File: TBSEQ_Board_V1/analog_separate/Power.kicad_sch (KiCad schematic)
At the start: 7 parts, among them IC11 AN6562, IC12 4066, J1 Conn_01x03_Pin, J3 Conn_01x03_Pin, J4 Conn_01x03_Pin, J5 Conn_01x03_Pin, J6 Conn_01x03_Pin

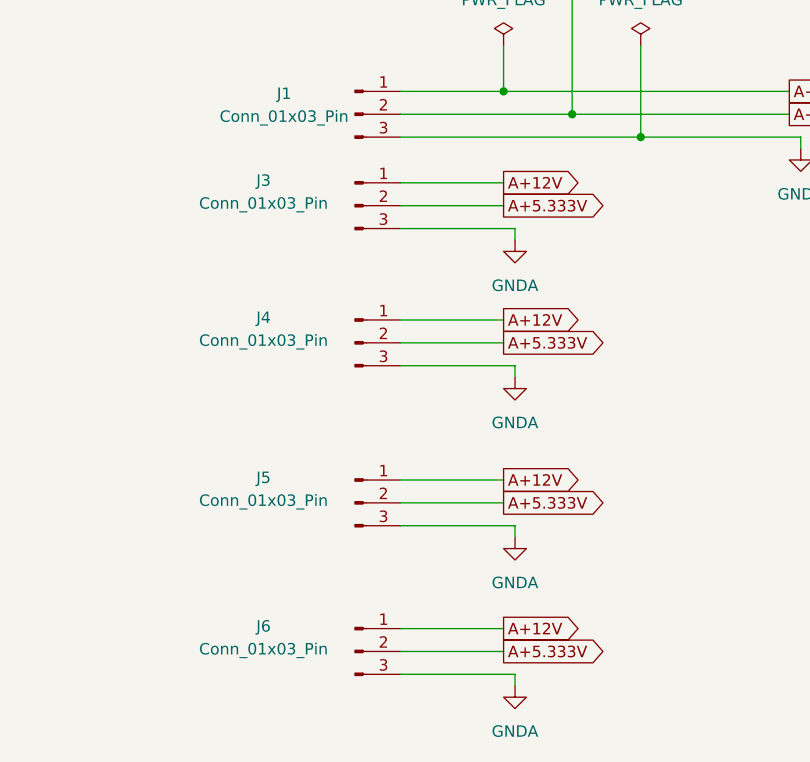
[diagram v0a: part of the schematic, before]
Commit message: replace
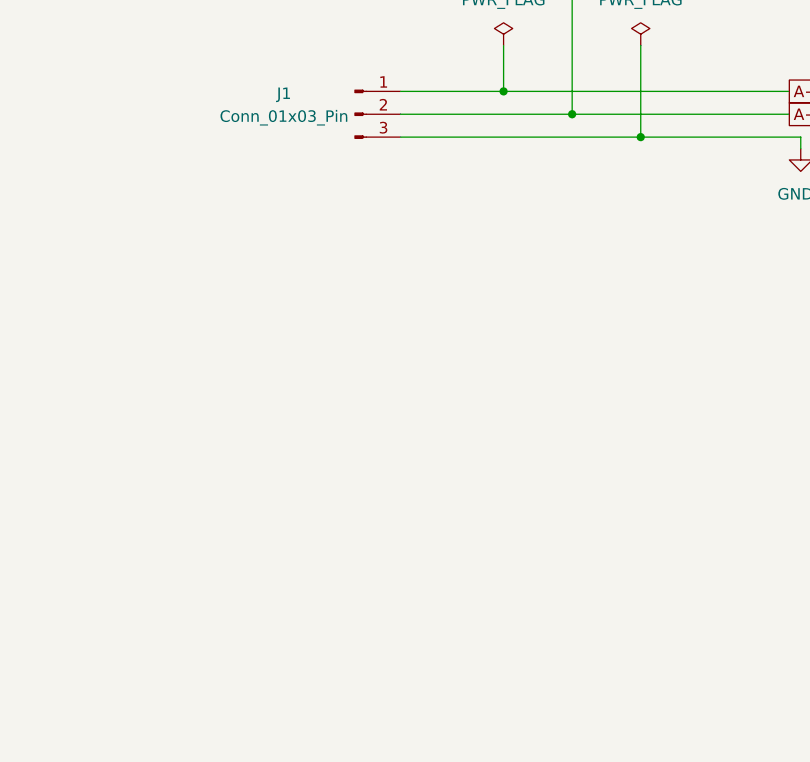
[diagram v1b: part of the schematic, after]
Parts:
- removed J3, J4, J5, J6: Conn_01x03_Pin, Connector_PinHeader_2.54mm:PinHeader_1x03_P2.54mm_Vertical, symbol Connector:Conn_01x03_Pin
